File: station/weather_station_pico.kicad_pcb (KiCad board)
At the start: 2 copper layers, 75.1 x 75 mm, 22 parts, among them J1 DebugHeader, J2 STEMMA_QT, J3 73412-0110, J4 STEMMA, J5 RJ11, J6 RJ11, J7 DS18B20, J8 Conn_01x04, U1 Pico, U2 RFM69

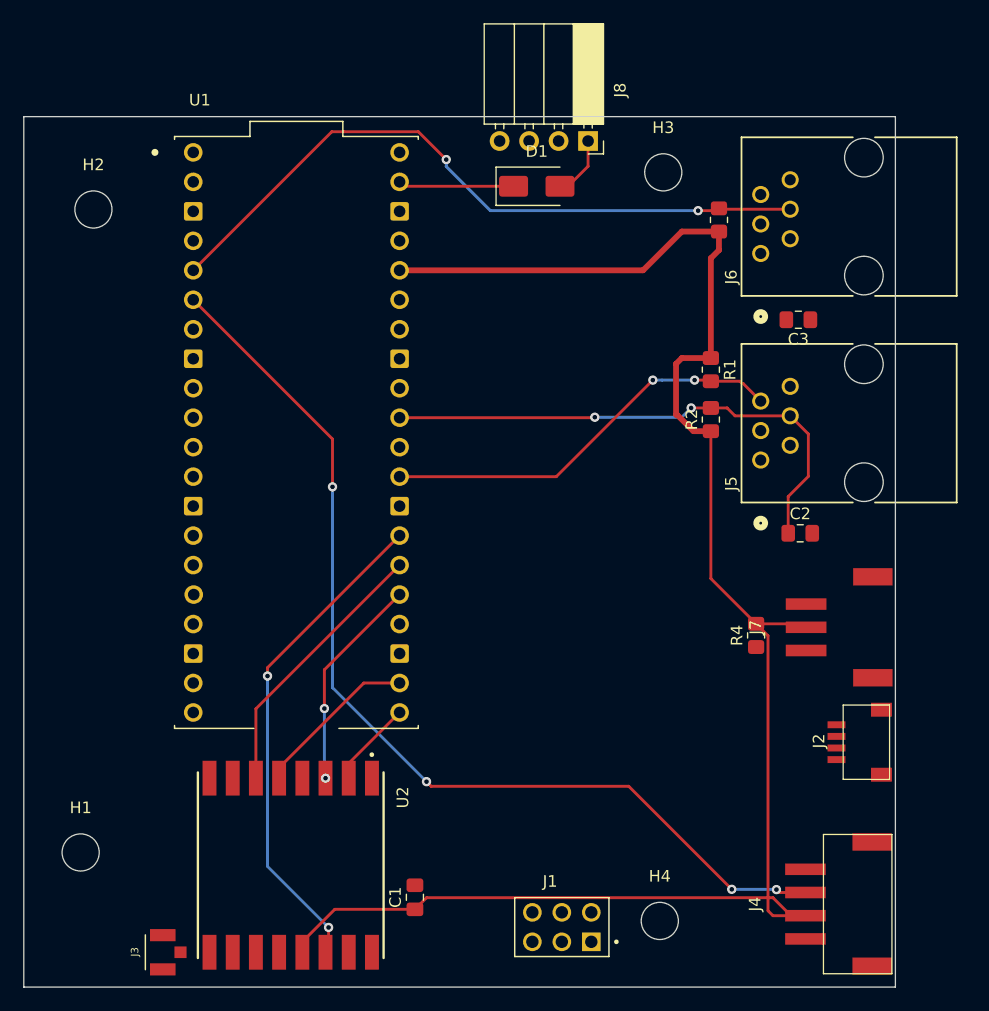
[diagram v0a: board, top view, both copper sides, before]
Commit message: Signed-off-by: Scott Perkins <whatisbyandby@gmail.com>
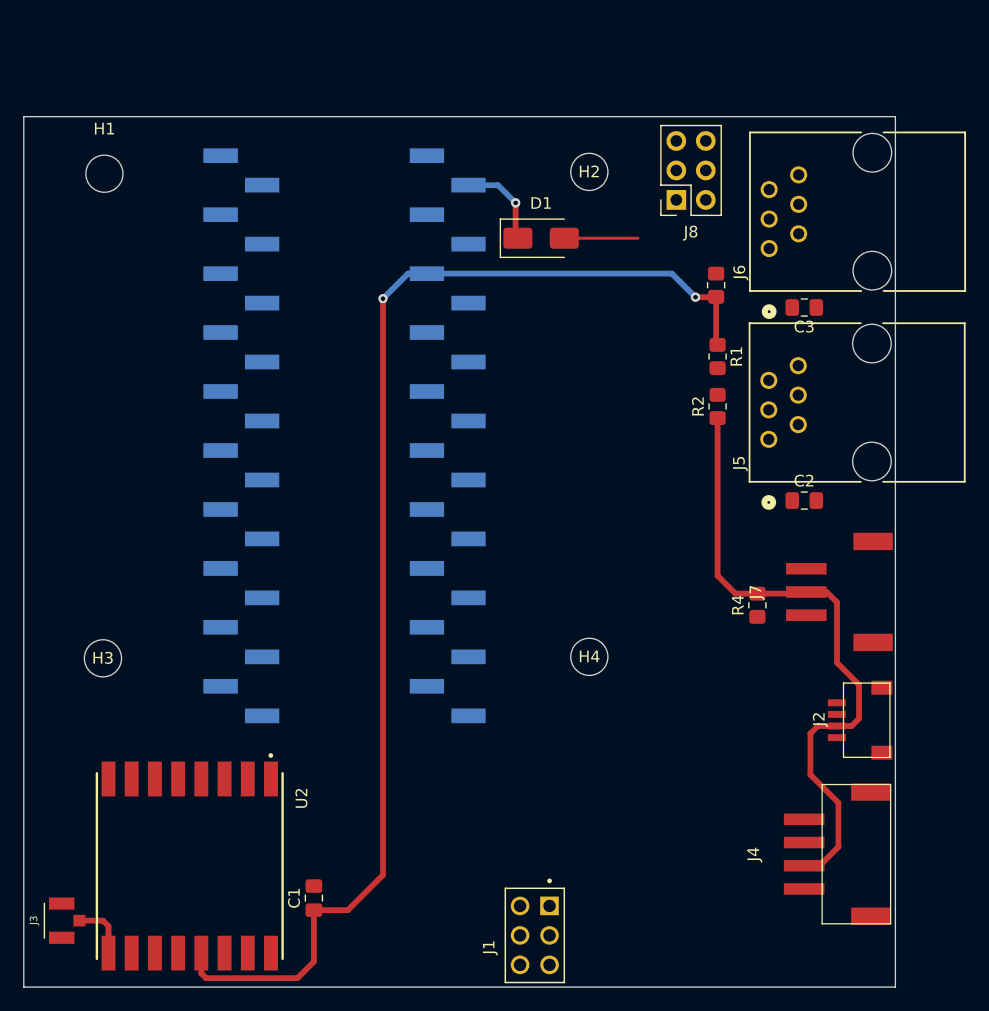
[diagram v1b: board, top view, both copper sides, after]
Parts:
- J8: value Conn_01x04 -> Battery Charger; footprint Connector_PinSocket_2.54mm:PinSocket_1x04_P2.54mm_Horizontal -> Connector_PinSocket_2.54mm:PinSocket_2x03_P2.54mm_Vertical
- U1: footprint WeatherStation:MODULE_SC918_PINS -> WeatherStation:Pico_SMD_Headers; moved to B.Cu
- moved H3 63.9 mm to (117.2, 106.2)
- moved H1 58.5 mm to (117.3, 64.4)
- moved H2 42.9 mm to (159.1, 64.3)
- moved H4 23.6 mm to (159.1, 106.0)
- moved J8 9.14 mm to (166.6, 66.7), turned to 180 degrees
- moved J3 9.12 mm to (113.7, 128.8)
- moved U2 8.70 mm to (124.7, 124.1)
- moved C1 8.70 mm to (135.4, 126.8)
- moved R3 5.63 mm to (170.1, 74.0)
- moved D1 4.49 mm to (155.0, 70.0)
- moved U1 4.44 mm to (138.0, 88.3), turned to 180 degrees
- moved J4 4.30 mm to (179.4, 123.0)
- moved J7 3.04 mm to (179.6, 100.5)
- moved C2 2.84 mm to (177.7, 92.6)
- moved R4 2.60 mm to (173.6, 101.6)
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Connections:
- net /Battery Charger/VOUT renamed /Battery Charger/Load+
- J8 pad 2: /Battery Charger/SET -> GND
- J8 pad 3: /Battery Charger/~{FAULT} -> GND
- J8 pad 4: /Battery Charger/~{CHRG} -> /Battery Charger/SET
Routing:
- net /I2C0_SDA: track 86.5 -> 0.00 mm, vias 4 -> 0
- net /RAIN_COUNT: track 59.7 -> 0.00 mm, vias 2 -> 0
- net /WINDSPEED_TGR: track 45.8 -> 0.00 mm, vias 2 -> 0
- net /RFM69 Radio/RFM69_INTR: track 42.9 -> 0.00 mm, vias 2 -> 0
- net /WINDDIR_OUT: track 35.3 -> 0.00 mm, vias 2 -> 0
- net /RFM69 Radio/RFM69_RESET: track 23.5 -> 0.00 mm
- net /RFM69 Radio/RFM69_MOSI: track 18.5 -> 0.00 mm, vias 2 -> 0
- net /RFM69 Radio/RFM69_CS: track 14.3 -> 0.00 mm
- net +3.3V: track 148.9 -> 163.0 mm, vias 0 -> 2
- net /RFM69 Radio/RFM69_MISO: track 7.47 -> 0.00 mm
- net Net-(U2-ANT): track 0.00 -> 5.01 mm
- net Net-(D1-K): track 9.98 -> 7.82 mm, vias 0 -> 1
- net /Battery Charger/Load+: track 5.31 -> 6.35 mm
